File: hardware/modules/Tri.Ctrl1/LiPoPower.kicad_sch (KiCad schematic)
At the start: 42 parts, among them J501 LiPo, SW501 Power Switch, U501 MCP73871-1CC, U502 INA226, U503 INA226, U504 TPS63070RNMR, U505 INA226

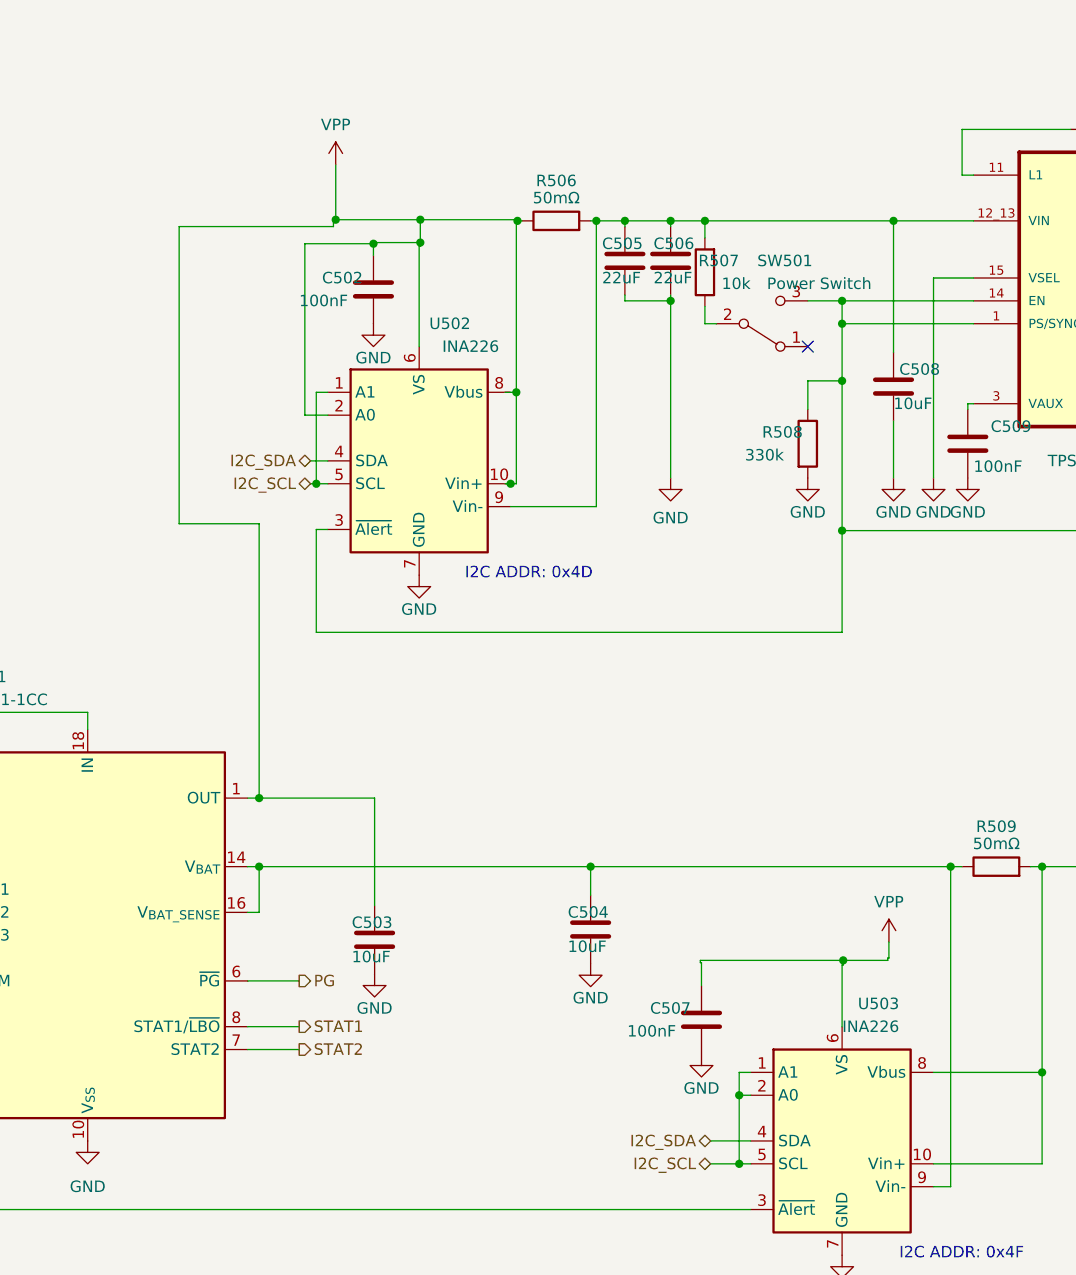
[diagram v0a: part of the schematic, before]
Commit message: 一通り配置
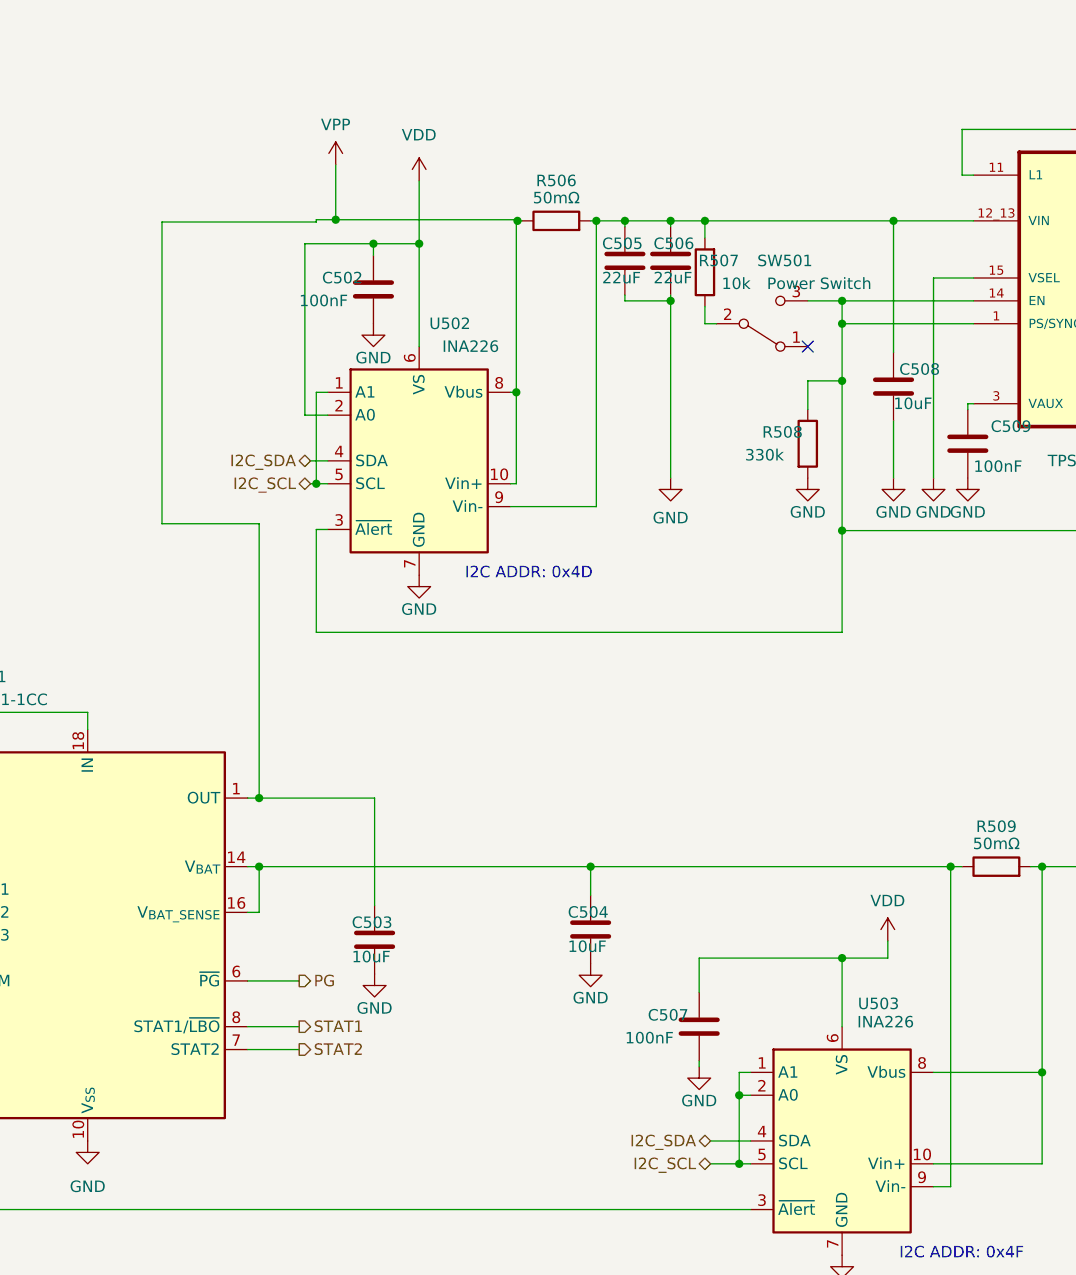
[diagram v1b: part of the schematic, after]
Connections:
- net VDD: now also C502.1, C507.1, U502.2 (A0), U502.6 (VS), U503.6 (VS)
- net VPP: now also U502.8 (Vbus); no longer C502.1, C507.1, U502.2 (A0), U502.6 (VS), U503.6 (VS)
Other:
- moved on the sheet: C507
